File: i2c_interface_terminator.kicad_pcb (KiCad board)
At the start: 2 copper layers, 15 x 11 mm, 0 parts

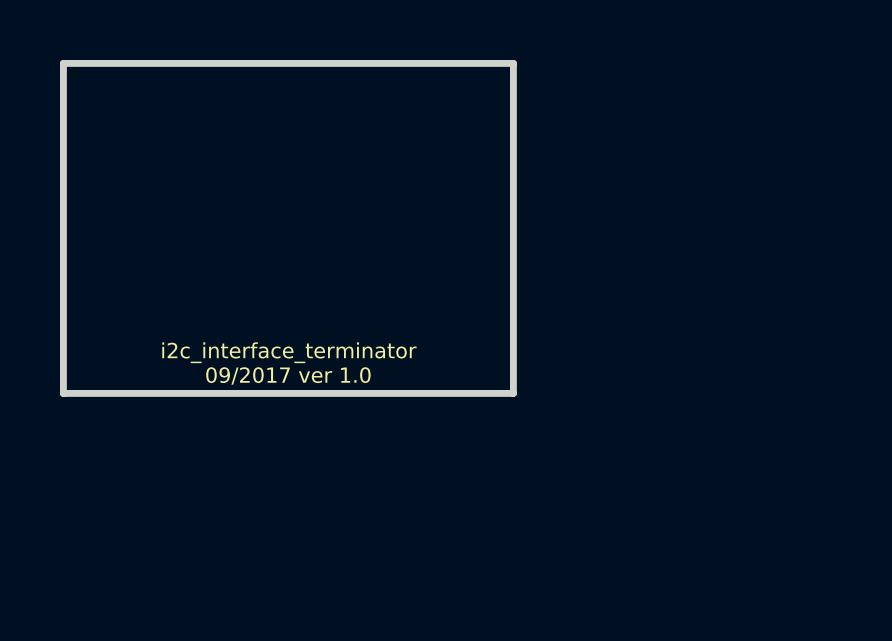
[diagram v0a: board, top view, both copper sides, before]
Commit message: Finished version 1.0.
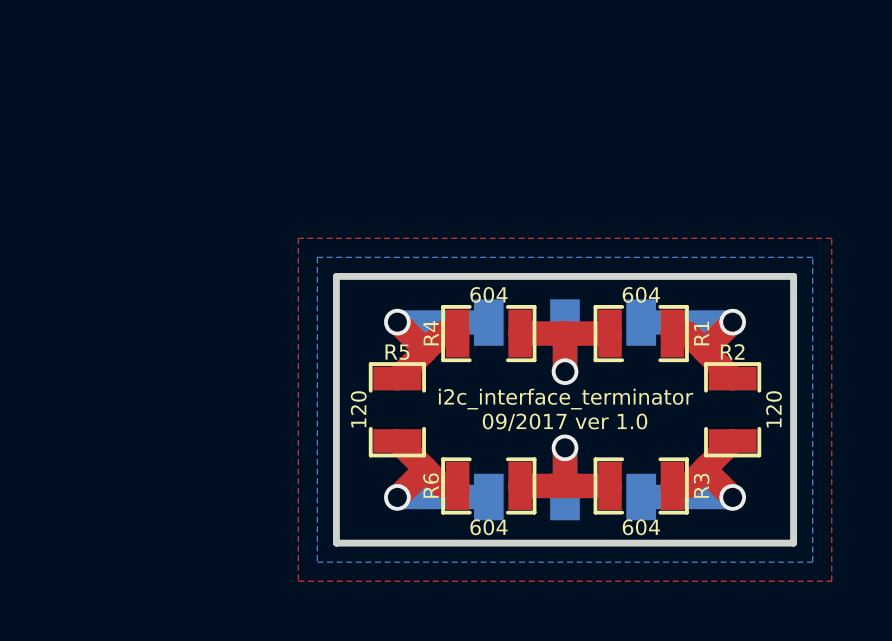
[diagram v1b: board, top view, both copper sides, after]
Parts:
- added P1: HEADER_02X03_FEMALE_SMD, i2c_interface_terminator:HEADER_02x03_FEMALE_SMD, B.Cu at (109.2, 106.0)
- added R1: 604, i2c_interface_terminator:SM0805, F.Cu at (111.8, 103.5)
- added R2: 120, i2c_interface_terminator:SM0805, F.Cu at (114.8, 106.0)
- added R3: 604, i2c_interface_terminator:SM0805, F.Cu at (111.8, 108.6)
- added R4: 604, i2c_interface_terminator:SM0805, F.Cu at (106.7, 103.5)
- added R5: 120, i2c_interface_terminator:SM0805, F.Cu at (103.6, 106.0)
- added R6: 604, i2c_interface_terminator:SM0805, F.Cu at (106.7, 108.6)
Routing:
- net /DSCLP: track 0.00 -> 7.18 mm, vias 0 -> 1
- net /DSCLM: track 0.00 -> 7.18 mm, vias 0 -> 1
- net /DSDAM: track 0.00 -> 7.18 mm, vias 0 -> 1
- net /DSDAP: track 0.00 -> 7.05 mm, vias 0 -> 1
- net VAA: track 0.00 -> 6.16 mm, vias 0 -> 1
- net GND: track 0.00 -> 5.91 mm, vias 0 -> 1
- added copper zone on B.Cu, net GND
- added copper zone on F.Cu, net VAA
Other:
- board size 15 x 11 mm -> 15.2 x 8.9 mm
- net class Default: trace_width 0.25 -> 0.254
